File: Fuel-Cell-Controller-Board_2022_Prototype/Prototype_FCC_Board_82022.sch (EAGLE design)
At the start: 148 parts, among them IC1 MAX232ECWE, IC2 TLV2404IN, IC3 TLV2404IN, J1 RJ45_LED, J10 RJ45_LED, J2 BLUETOOTH, J3 RJ45_LED, J4 RJ45_LED, J5 RJ45_LED, J6 RJ45_LED, J7 RJ45_LED, J8 RJ45_LED, J9 RJ45_LED

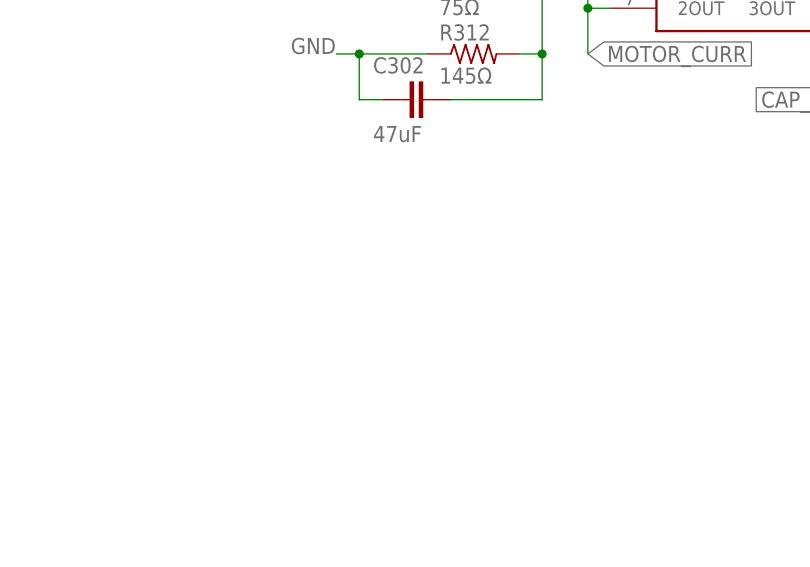
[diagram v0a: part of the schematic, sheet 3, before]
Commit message: new resistor
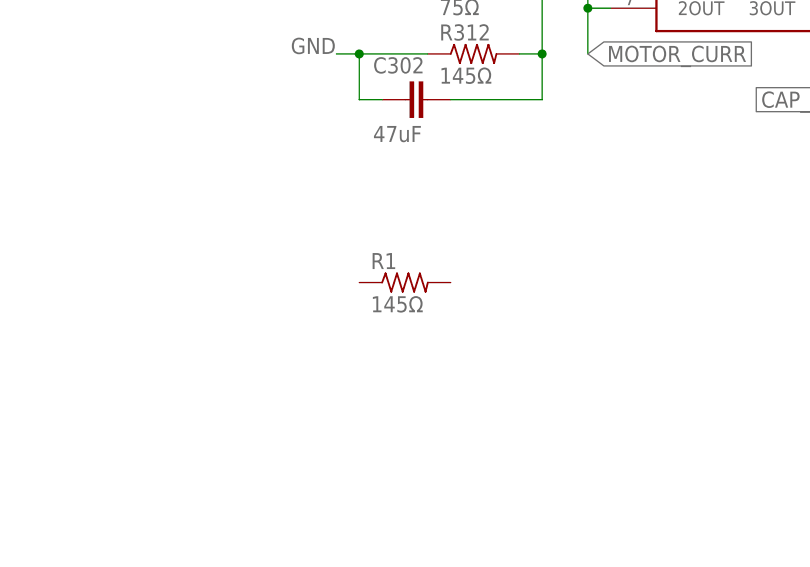
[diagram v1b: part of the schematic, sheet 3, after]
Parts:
- added R1: 145Ω, resistor:R-US_R0805
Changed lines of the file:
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@@
 <part name="GND26" library="E-P-008-R1.2" deviceset="GND" device=""/>
 <part name="D308" library="12V TVS" deviceset="P6KE15A-E3/54GICT-ND" device=""/>
+<part name="R1" library="resistor" library_urn="urn:adsk.eagle:library:348" deviceset="R-US_" device="R0805" package3d_urn="urn:adsk.eagle:package:26059/1" value="145Ω"/>
 </parts>
 <sheets>
@@
 <attribute name="VALUE" x="63.4746" y="81.8642" size="1.778" layer="96"/>
 </instance>
+<instance part="R1" gate="G$1" x="157.48" y="48.26" smashed="yes">
+<attribute name="NAME" x="153.67" y="49.7586" size="1.778" layer="95"/>
+<attribute name="VALUE" x="153.67" y="44.958" size="1.778" layer="96"/>
+</instance>
 </instances>

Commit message: update
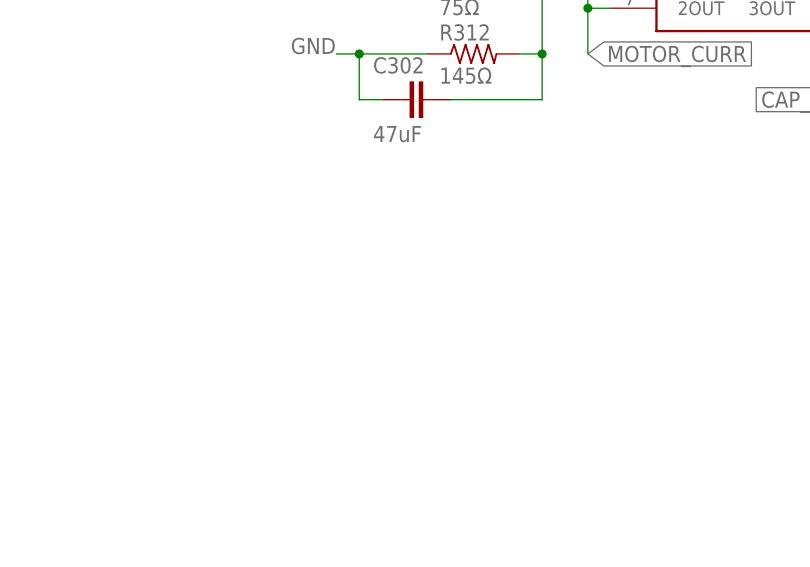
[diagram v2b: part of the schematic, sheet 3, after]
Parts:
- removed R1: 145Ω, resistor:R-US_R0805
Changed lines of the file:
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@@
 <part name="GND26" library="E-P-008-R1.2" deviceset="GND" device=""/>
 <part name="D308" library="12V TVS" deviceset="P6KE15A-E3/54GICT-ND" device=""/>
-<part name="R1" library="resistor" library_urn="urn:adsk.eagle:library:348" deviceset="R-US_" device="R0805" package3d_urn="urn:adsk.eagle:package:26059/1" value="145Ω"/>
 </parts>
 <sheets>
@@
 <attribute name="VALUE" x="63.4746" y="81.8642" size="1.778" layer="96"/>
 </instance>
-<instance part="R1" gate="G$1" x="157.48" y="48.26" smashed="yes">
-<attribute name="NAME" x="153.67" y="49.7586" size="1.778" layer="95"/>
-<attribute name="VALUE" x="153.67" y="44.958" size="1.778" layer="96"/>
-</instance>
 </instances>
